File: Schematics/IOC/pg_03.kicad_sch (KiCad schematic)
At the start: 2 parts

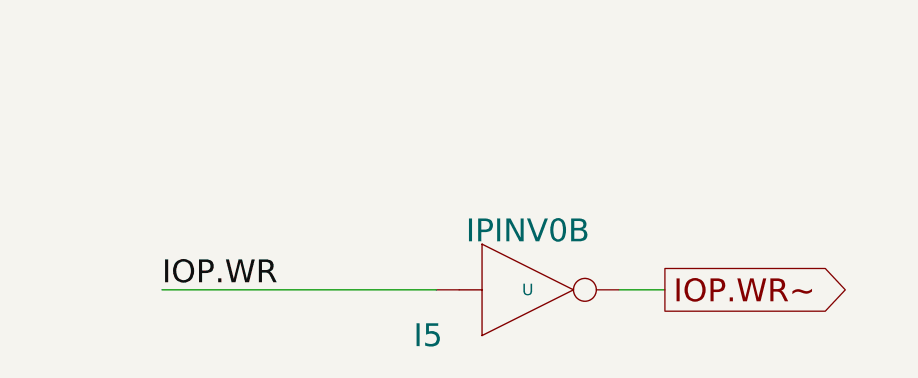
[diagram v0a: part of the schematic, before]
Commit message: Tested to 21.6 seconds (rm073)
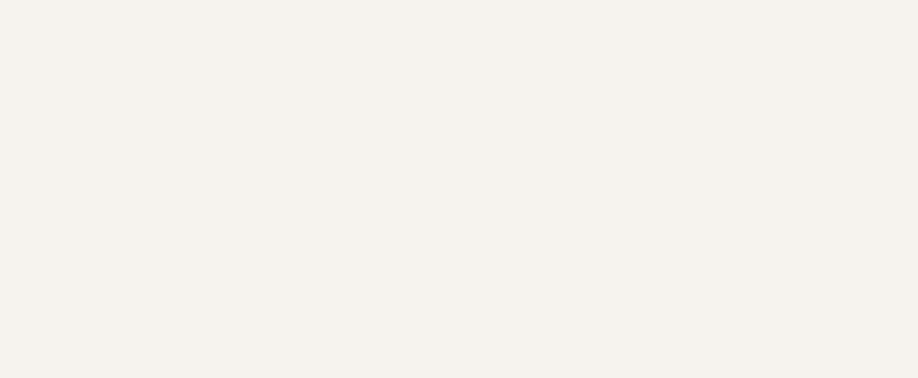
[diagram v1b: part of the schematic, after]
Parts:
- removed U: (no value), symbol r1000:F04
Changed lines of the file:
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@@
     (comment 4 "RELEASED")
-  )
-  (wire (pts (xy 213.36 40.64) (xy 218.44 40.64))
-    (stroke (width 0) (type default))
-  )
-  (wire (pts (xy 162.56 40.64) (xy 193.04 40.64))
-    (stroke (width 0) (type default))
   )
   (wire (pts (xy 78.74 17.78) (xy 104.14 17.78))
@@
     (stroke (width 0) (type default))
   )
-  (label "IOP.WR" (at 162.56 40.64 0) (fields_autoplaced)
-    (effects (font (size 2.54 2.54)) (justify left bottom))
-  )
   (global_label "WR~" (shape input) (at 40.64 17.78 180) (fields_autoplaced)
     (effects (font (size 2.54 2.54)) (justify right))
     (property "Intersheet References" "${INTERSHEET_REFS}" (id 0) (at 28.1759 17.6213 0)
       (effects (font (size 1.905 1.905)) (justify right))
-    )
-  )
-  (global_label "IOP.WR~" (shape output) (at 218.44 40.64 0) (fields_autoplaced)
-    (effects (font (size 2.54 2.54)) (justify left))
-    (property "Intersheet References" "${INTERSHEET_REFS}" (id 0) (at 238.5241 40.4813 0)
-      (effects (font (size 1.905 1.905)) (justify left))
     )
   )
@@
     )
   )
-  (symbol (lib_id "r1000:F04") (at 203.2 40.64 0) (unit 1)
-    (in_bom yes) (on_board yes)
-    (default_instance (reference "U") (unit 1) (value "") (footprint ""))
-    (property "Reference" "U" (id 0) (at 203.2 40.64 0)
-      (effects (font (size 1.27 1.27)))
-    )
-    (property "Value" "" (id 1) (at 204.47 45.72 0)
-      (effects (font (size 2.54 2.54)) (justify left))
-    )
-    (property "Footprint" "" (id 2) (at 203.2 40.64 0)
-      (effects (font (size 1.27 1.27)) hide)
-    )
-    (property "Datasheet" "" (id 3) (at 203.2 40.64 0)
-      (effects (font (size 1.27 1.27)) hide)
-    )
-    (property "Location" "I5" (id 4) (at 190.5 45.72 0)
-      (effects (font (size 2.54 2.54)) (justify left))
-    )
-    (property "Name" "IPINV0B" (id 5) (at 203.2 35.56 0)
-      (effects (font (size 2.54 2.54)) (justify bottom))
-    )
-    (pin "1")
-    (pin "2")
-  )
   (symbol (lib_id "r1000:F04") (at 68.58 17.78 0) (unit 1)
